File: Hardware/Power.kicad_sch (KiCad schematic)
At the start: 0 parts

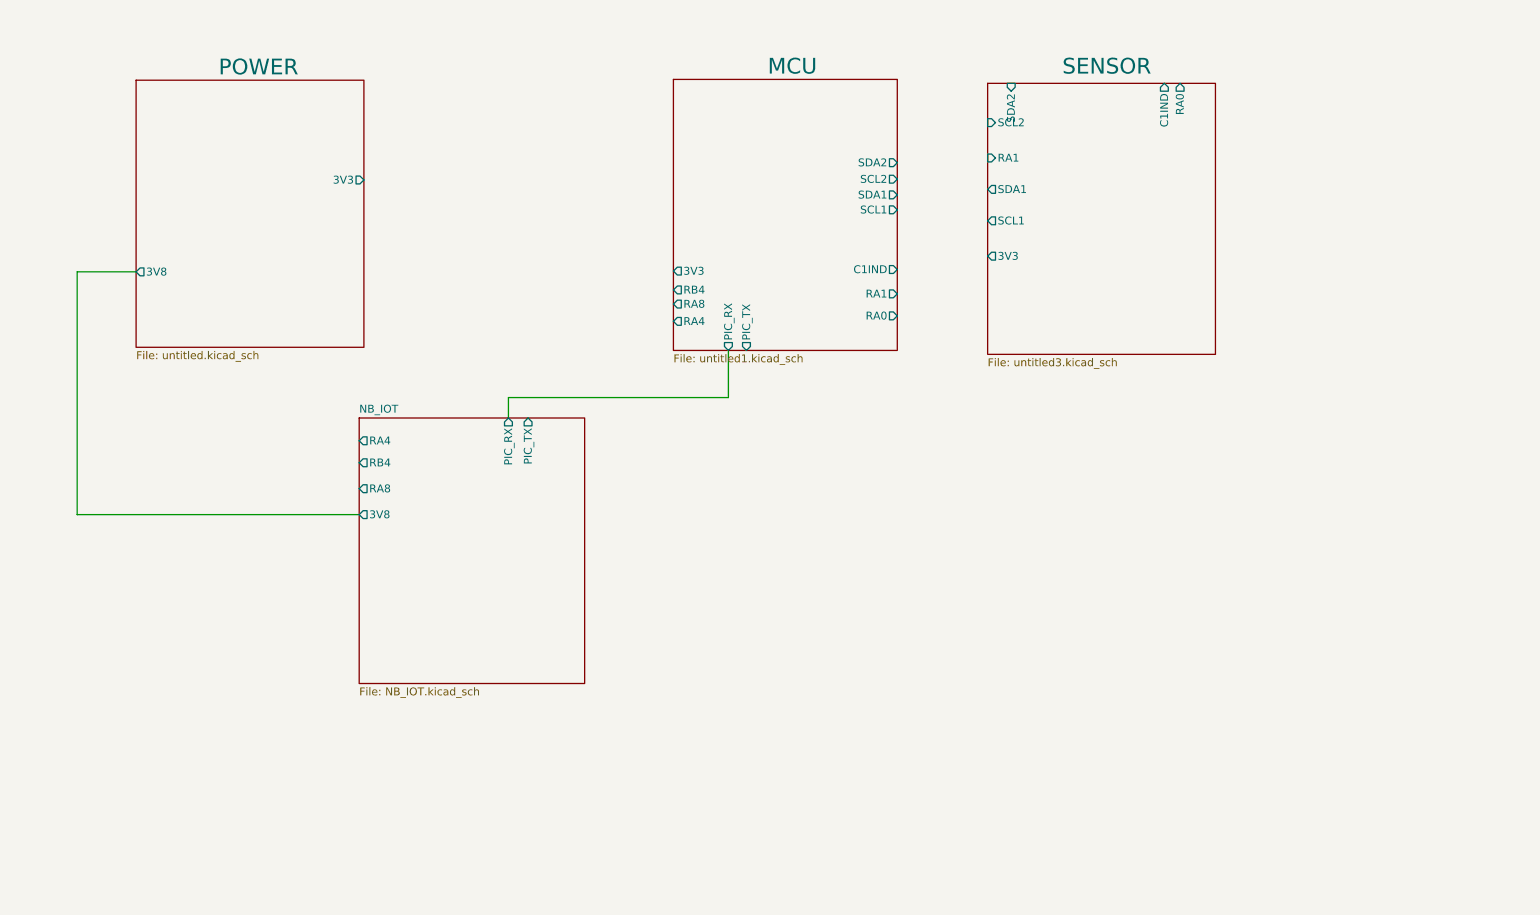
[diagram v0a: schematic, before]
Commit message: FIX
fix
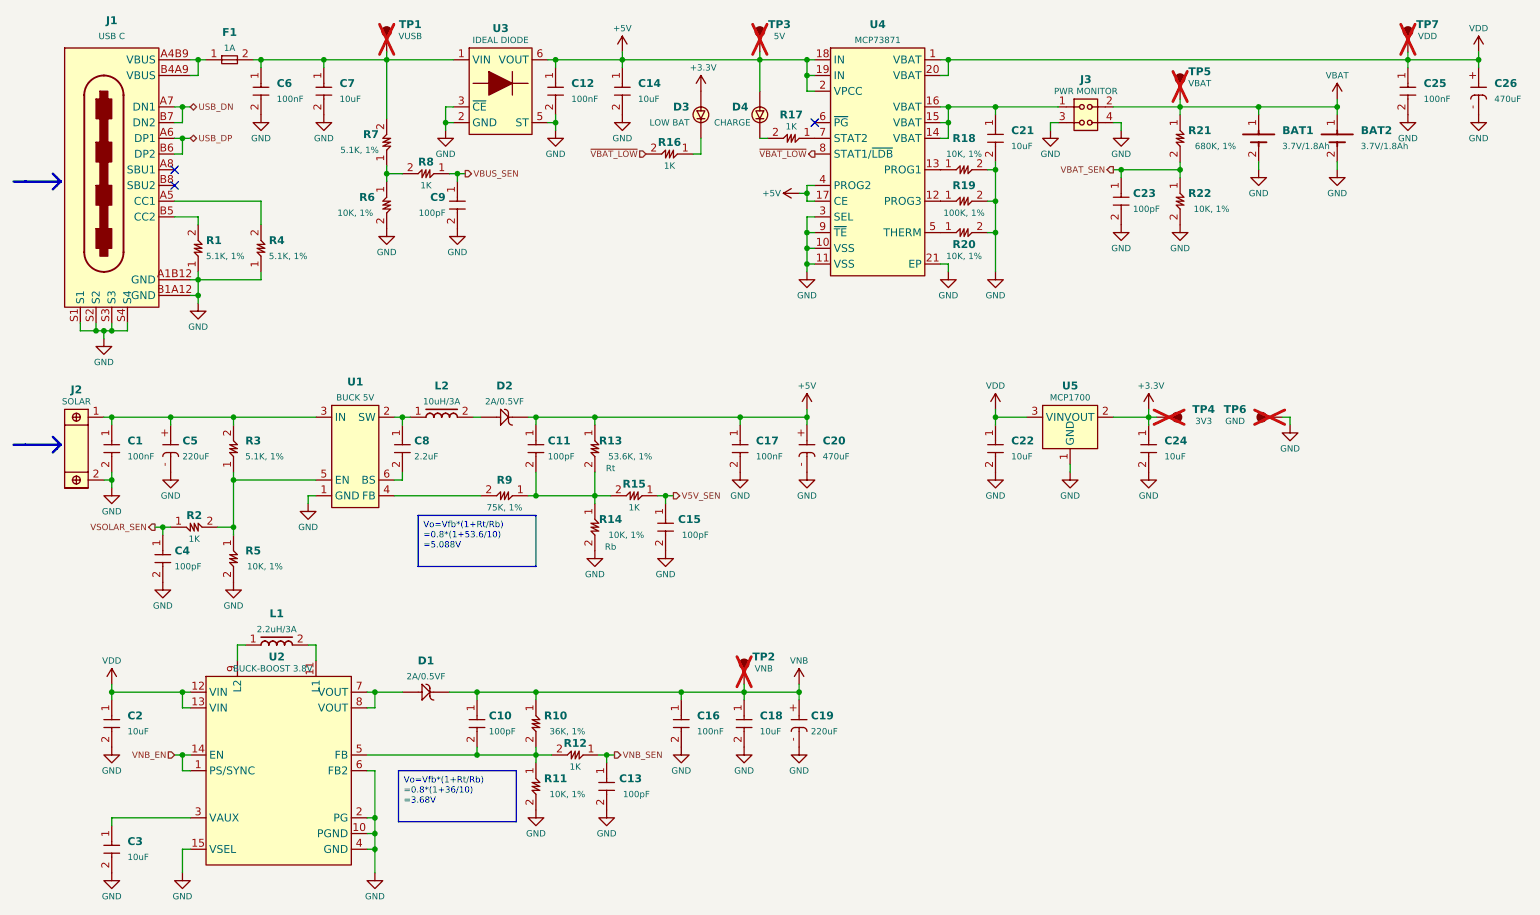
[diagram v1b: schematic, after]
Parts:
- added BAT1, BAT2: 3.7V/1.8Ah, symbol SAMPI:BATTERY
- added C1, C12, C16, C17, C25, C6: 100nF, SAMPI:CAP0603, symbol SAMPI:CERCAP
- added C10, C11, C13, C15, C23, C4, C9: 100pF, SAMPI:CAP0603, symbol SAMPI:CERCAP
- added C14, C18, C2, C21, C22, C24, C3, C7: 10uF, SAMPI:CAP0805, symbol SAMPI:CERCAP
- added C19, C5: 220uF, symbol SAMPI:ELECCAP
- added C20, C26: 470uF, symbol SAMPI:ELECCAP
- added C8: 2.2uF, SAMPI:CAP0603, symbol SAMPI:CERCAP
- added D1, D2: 2A/0.5VF, symbol SAMPI:DIODE-SCH
- added D3: LOW BAT, SAMPI:LED0603, symbol SAMPI:RLED
- added D4: CHARGE, SAMPI:LED0603, symbol SAMPI:GLED
- added F1: 1A, symbol SAMPI:FUSE
- added J1: USB C, SAMPI:USB4105, symbol SAMPI:USB4105
- added J2: SOLAR, PAD02_2.54TH, symbol SAMPI:SIL02
- added J3: PWR MONITOR, symbol SAMPI:DIL04
- added L1: 2.2uH/3A, symbol SAMPI:IND_HC
- added L2: 10uH/3A, symbol SAMPI:IND_HC
- added R1, R3, R4, R7: 5.1K, 1%, SAMPI:RES0603, symbol SAMPI:RES
- added R10: 36K, 1%, SAMPI:RES0603, symbol SAMPI:RES
- added R11, R14, R18, R20, R22, R5, R6: 10K, 1%, SAMPI:RES0603, symbol SAMPI:RES
- added R12, R15, R16, R17, R2, R8: 1K, SAMPI:RES0603, symbol SAMPI:RES
- added R13: 53.6K, 1%, SAMPI:RES0603, symbol SAMPI:RES
- added R19: 100K, 1%, SAMPI:RES0603, symbol SAMPI:RES
- added R21: 680K, 1%, SAMPI:RES0603, symbol SAMPI:RES
- added R9: 75K, 1%, SAMPI:RES0603, symbol SAMPI:RES
- added TP1: VUSB, symbol SAMPI:TESTPOINT
- added TP2: VNB, symbol SAMPI:TESTPOINT
- added TP3: 5V, symbol SAMPI:TESTPOINT
- added TP4: 3V3, symbol SAMPI:TESTPOINT
- added TP5: VBAT, symbol SAMPI:TESTPOINT
- added TP6: GND, symbol SAMPI:TESTPOINT
- added TP7: VDD, symbol SAMPI:TESTPOINT
- added U1: BUCK 5V, SAMPI:SOT-23-6_MCHP, symbol SAMPI:MP1470
- added U2: BUCK-BOOST 3.8V, symbol SAMPI:TPS630701
- added U3: IDEAL DIODE, SAMPI:SOT363, symbol SAMPI:DIODE_IDEAL_LM66100
- added U4: MCP73871, symbol SAMPI:MCP73871
- added U5: MCP1700, SAMPI:SOT23, symbol SAMPI:LDO
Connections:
- new net: C6.1, C7.1, F1.2, R7.2, TP1.1, U3.1 (VIN)
- new net: C11.2, R13.2, R14.1, R15.2, R9.1
- new net: R18.1, U4.13 (PROG1)
- new net: L1.1, U2.9 (L2)
- new net: L1.2, U2.11 (L1)
- new net: C3.1, U2.3 (VAUX)
- new net: C10.2, R10.2, R11.1, R12.2, U2.5 (FB)
- new net: D1.A, U2.7 (VOUT), U2.8 (VOUT)
- new net: C8.1, L2.1, U1.2 (SW)
- new net: C8.2, U1.6 (BS)
- new net: R20.1, U4.5 (THERM)
- new net: D2.A, L2.2
- new net: R9.2, U1.4 (FB)
- new net: R17.1, U4.7 (STAT2)
- new net: D4.K, R17.2
- new net: J1.B5 (CC2), R1.2
- new net: R2.2, R3.1, R5.1, U1.5 (EN)
- new net: C21.1, J3.1, U4.14 (VBAT), U4.15 (VBAT), U4.16 (VBAT)
- new net: F1.1, J1.A4B9 (VBUS), J1.B4A9 (VBUS)
- new net: J1.A5 (CC1), R4.2
- new net: C1.1, C5.+, J2.1, R3.2, U1.3 (IN)
- new net: R6.1, R7.1, R8.2
- new net: R19.1, U4.12 (PROG3)
- new net: D3.K, R16.1
- new net +3.3V: C24.1, D3.A, TP4.1, U5.2 (VOUT)
- new net +5V: C11.1, C12.1, C14.1, C17.1, C20.+, D2.K, D4.A, R13.1, TP3.1, U3.6 (VOUT), U4.17 (CE), U4.18 (IN), U4.19 (IN), U4.2 (VPCC), U4.4 (PROG2)
- new net GND: BAT1.2 (-), BAT2.2 (-), C1.2, C12.2, C13.2, C14.2, C15.2, C16.2, C17.2, C18.2, C19.-, C2.2, C20.-, C21.2, C22.2, C23.2, C24.2, C25.2, C26.-, C3.2, C4.2, C5.-, C6.2, C7.2, C9.2, J1.A1B12 (GND), J1.B1A12 (GND), J1.S1, J1.S2, J1.S3, J1.S4, J2.2, J3.3, J3.4, R1.1, R11.2, R14.2, R18.2, R19.2, R20.2, R22.2, R4.1, R5.2, R6.2, TP6.1, U1.1 (GND), U2.10 (PGND), U2.15 (VSEL), U2.2 (PG), U2.4 (GND), U2.6 (FB2), U3.2 (GND), U3.3 (~{CE}), U3.5 (ST), U4.10 (VSS), U4.11 (VSS), U4.21 (EP), U4.3 (SEL), U4.9 (~{TE}), U5.1 (GND)
- new net USB_DN: J1.A7 (DN1), J1.B7 (DN2)
- new net USB_DP: J1.A6 (DP1), J1.B6 (DP2)
- new net V5V_SEN: C15.1, R15.1
- new net VBAT: BAT1.1 (+), BAT2.1 (+), J3.2, R21.1, TP5.1
- new net VBAT_SEN: C23.1, R21.2, R22.1
- new net VBUS_SEN: C9.1, R8.1
- new net VDD: C2.1, C22.1, C25.1, C26.+, TP7.1, U2.12 (VIN), U2.13 (VIN), U4.1 (VBAT), U4.20 (VBAT), U5.3 (VIN)
- new net VNB: C10.1, C16.1, C18.1, C19.+, D1.K, R10.1, TP2.1
- new net VNB_EN: U2.1 (PS/SYNC), U2.14 (EN)
- new net VNB_SEN: C13.1, R12.1
- new net VSOLAR_SEN: C4.1, R2.1
- new net ~{VBAT_LOW}: R16.2, U4.8 (STAT1/~{LDB})
- no-connect marks 0 -> 3
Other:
- removed sheet MCU
- removed sheet NB_IOT
- removed sheet POWER
- removed sheet SENSOR
